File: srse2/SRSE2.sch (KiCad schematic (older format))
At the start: 64 parts, among them J1 S88, J2 CAN, P1 I2S, P10 PIC_SPARE, P11 RS485 TERM, P12 RS485, P13 CONN_01X03, P2 CONN_01X09, P3 opt 18V, P4 UART, P5 Grove, P6 ISO_I2C, P7 CAN_TERM, P8 CAN, P9 PIC_I2C, U1 Omega2, U2 ADuM1250CR, U3 MCP2562-I/SN, U4 PIC18F25K80, U5 HR911105A, U6 SP3485CN, U7 FT230XS, Y1 16MHz

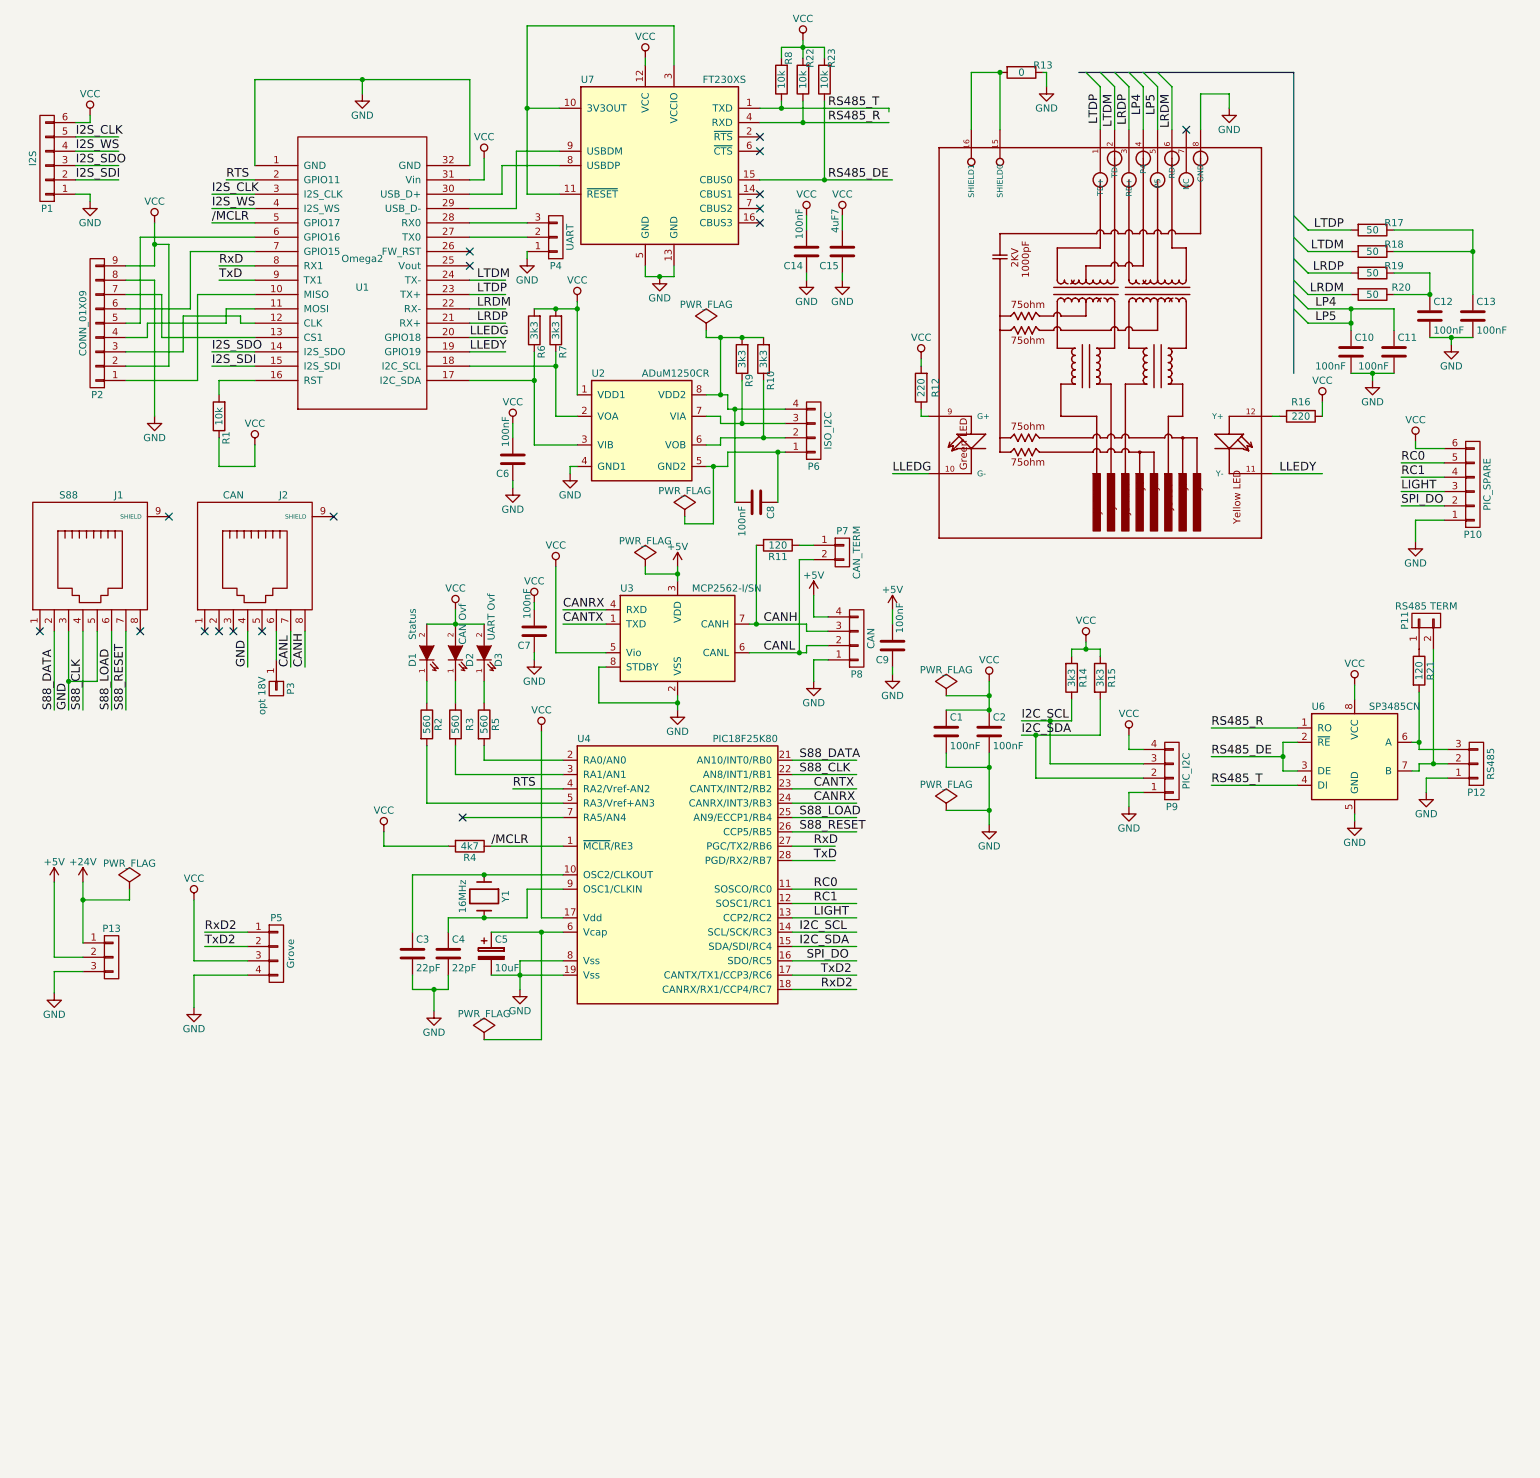
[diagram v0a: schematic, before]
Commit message: wip
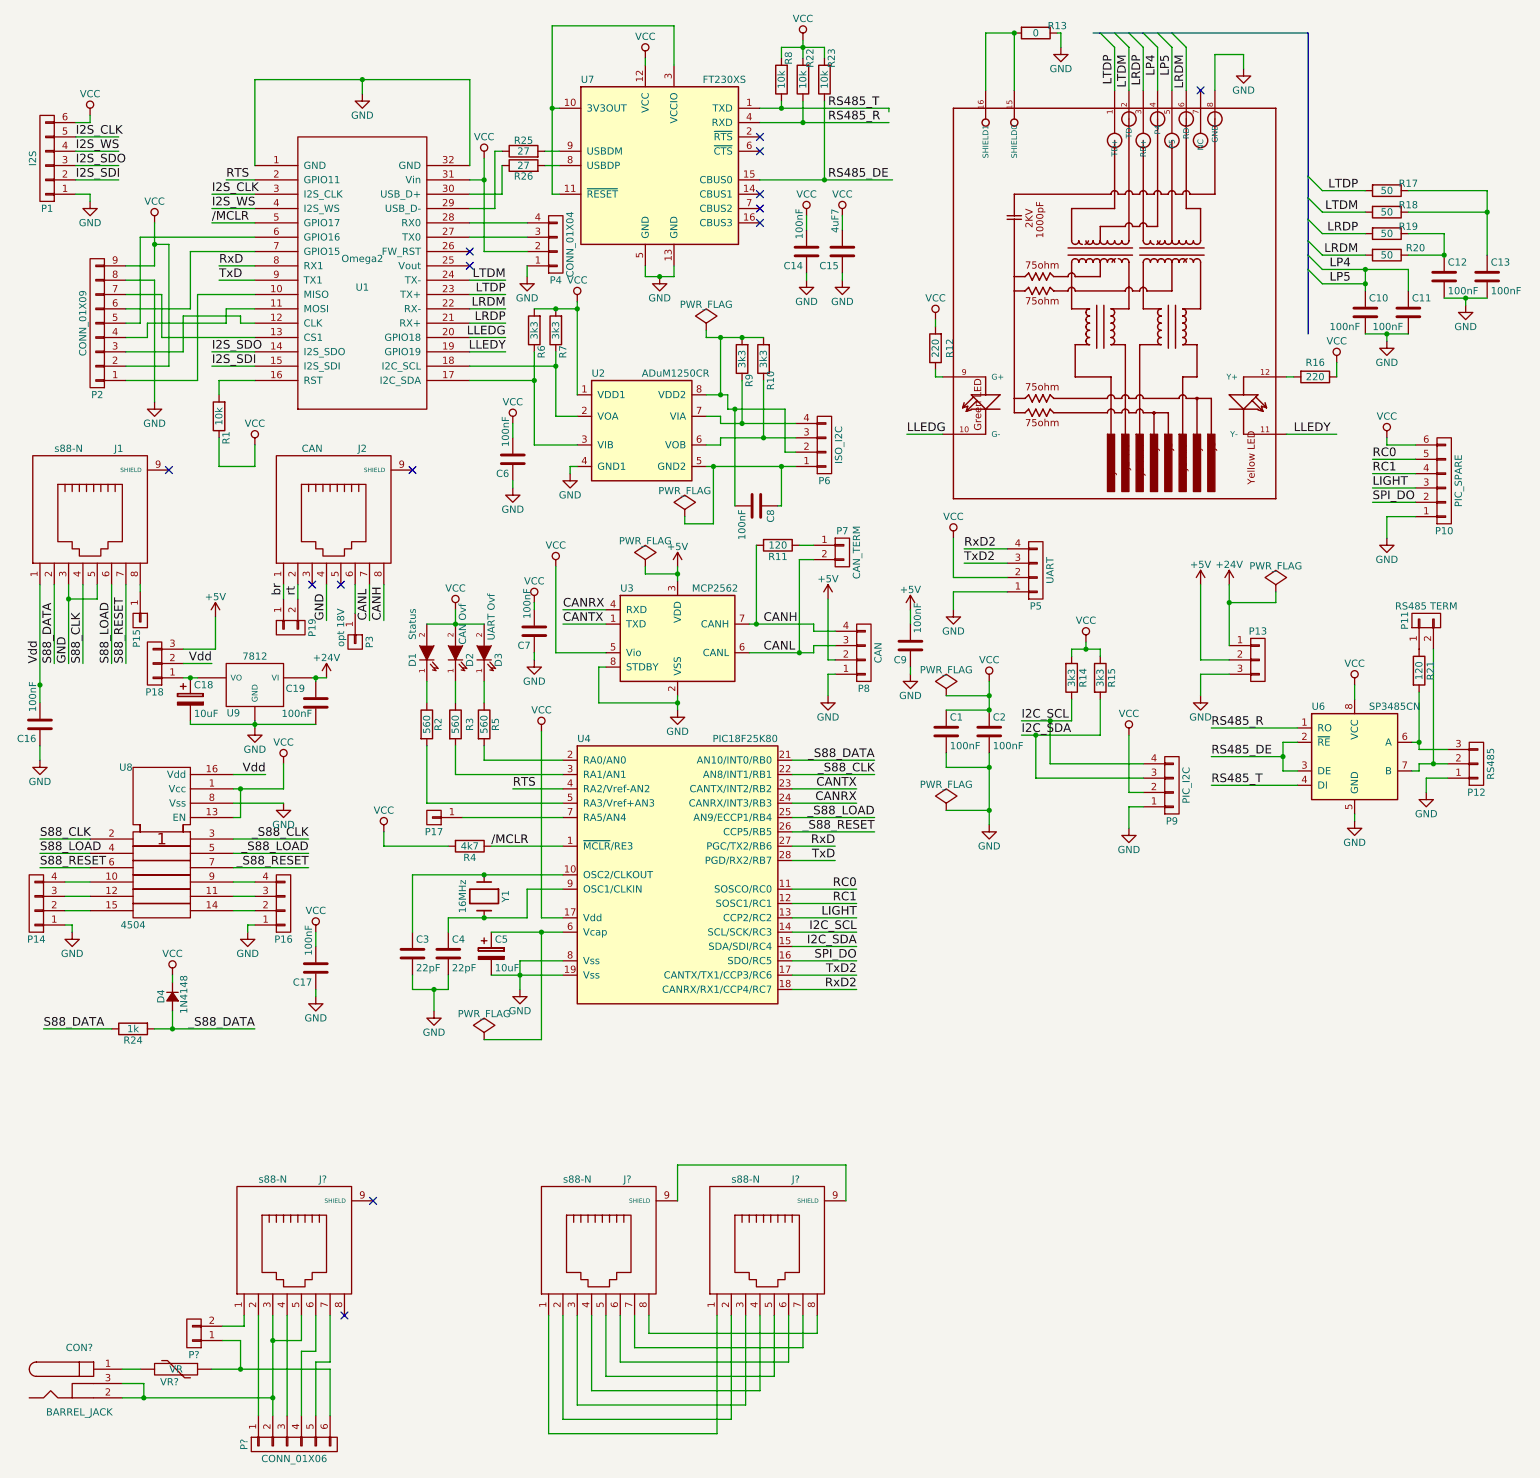
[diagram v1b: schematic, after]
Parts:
- removed P4: UART, Pin_Headers:Pin_Header_Straight_1x03, symbol CONN_01X03
- added C16, C17, C19: 100nF, Capacitors_SMD:C_0805_HandSoldering, symbol C
- added C18: 10uF, Capacitors_ThroughHole:C_Radial_D5_L6_P2.5, symbol CP
- added CON?: BARREL_JACK, symbol BARREL_JACK
- added D4: 1N4148, w_smd_diode:melf, symbol D_Small
- added J? (x3): s88-N, w_conn_pc:megb8-8, symbol RJ45
- added P14, P16: CONN_01X04, Pin_Headers:Pin_Header_Straight_1x04, symbol CONN_01X04
- added P15, P17: opt 18V, Pin_Headers:Pin_Header_Straight_1x01, symbol CONN_01X01
- added P18: CONN_01X03, Pin_Headers:Pin_Header_Angled_1x03, symbol CONN_01X03
- added P19, P?: CONN_01X02, Pin_Headers:Pin_Header_Straight_1x02, symbol CONN_01X02
- added P4: CONN_01X04, w_conn_jst-ph:b4b-ph-kl, symbol CONN_01X04
- added P?: CONN_01X06, symbol CONN_01X06
- added R24: 1k, Resistors_SMD:R_1206_HandSoldering, symbol R
- added R25, R26: 27, Resistors_SMD:R_0805_HandSoldering, symbol R
- added U8: 4504, w_smd_dil:so-16, symbol 4504
- added U9: 7812, TO_SOT_Packages_SMD:TO-252-2Lead, symbol 7805
- added VR?: VR, w_pth_resistors:RC07, symbol VR
- J1: value S88 -> s88-N
- P5: value Grove -> UART
- P6, P8, P9: footprint Pin_Headers:Pin_Header_Straight_1x04 -> w_conn_jst-ph:b4b-ph-kl
- U3: value MCP2562-I/SN -> MCP2562
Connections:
- net labels added: Vdd, _S88_CLK, _S88_DATA, _S88_LOAD, _S88_RESET, br, rt
- wire segments 320 -> 472
- no-connect marks 17 -> 14
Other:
- moved on the sheet: C10, C11, C12, C13, C8, C9, J1, J2, P10, P13, P3, P5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
